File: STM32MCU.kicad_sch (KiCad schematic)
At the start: 5 parts, among them U5 STM32C542CCT6

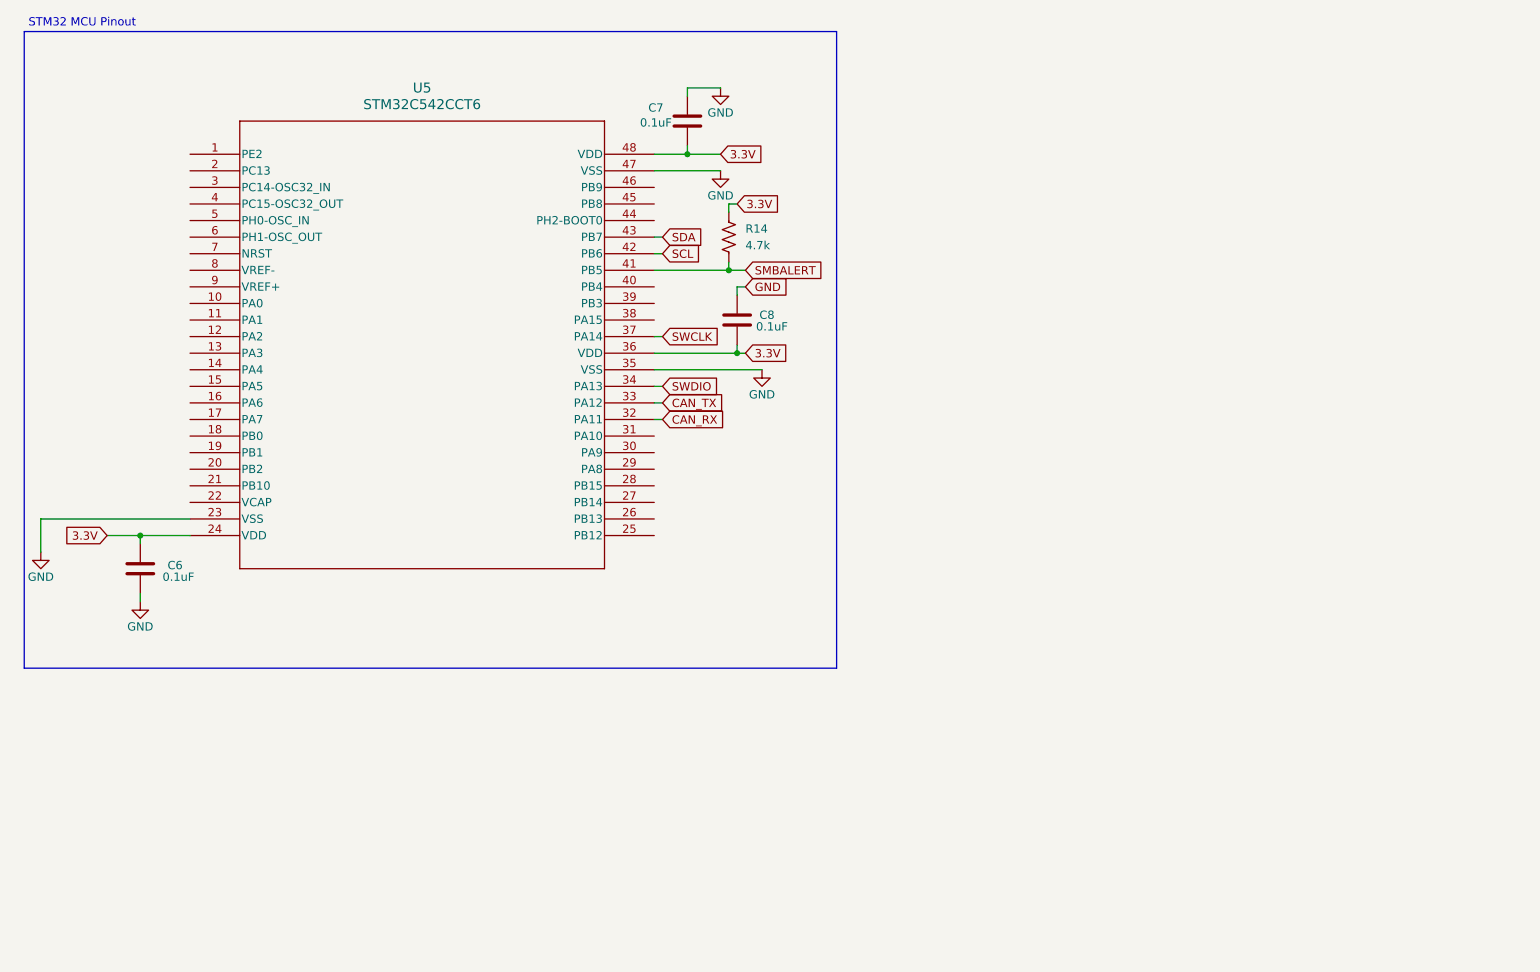
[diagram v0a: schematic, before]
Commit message: Updated MCU
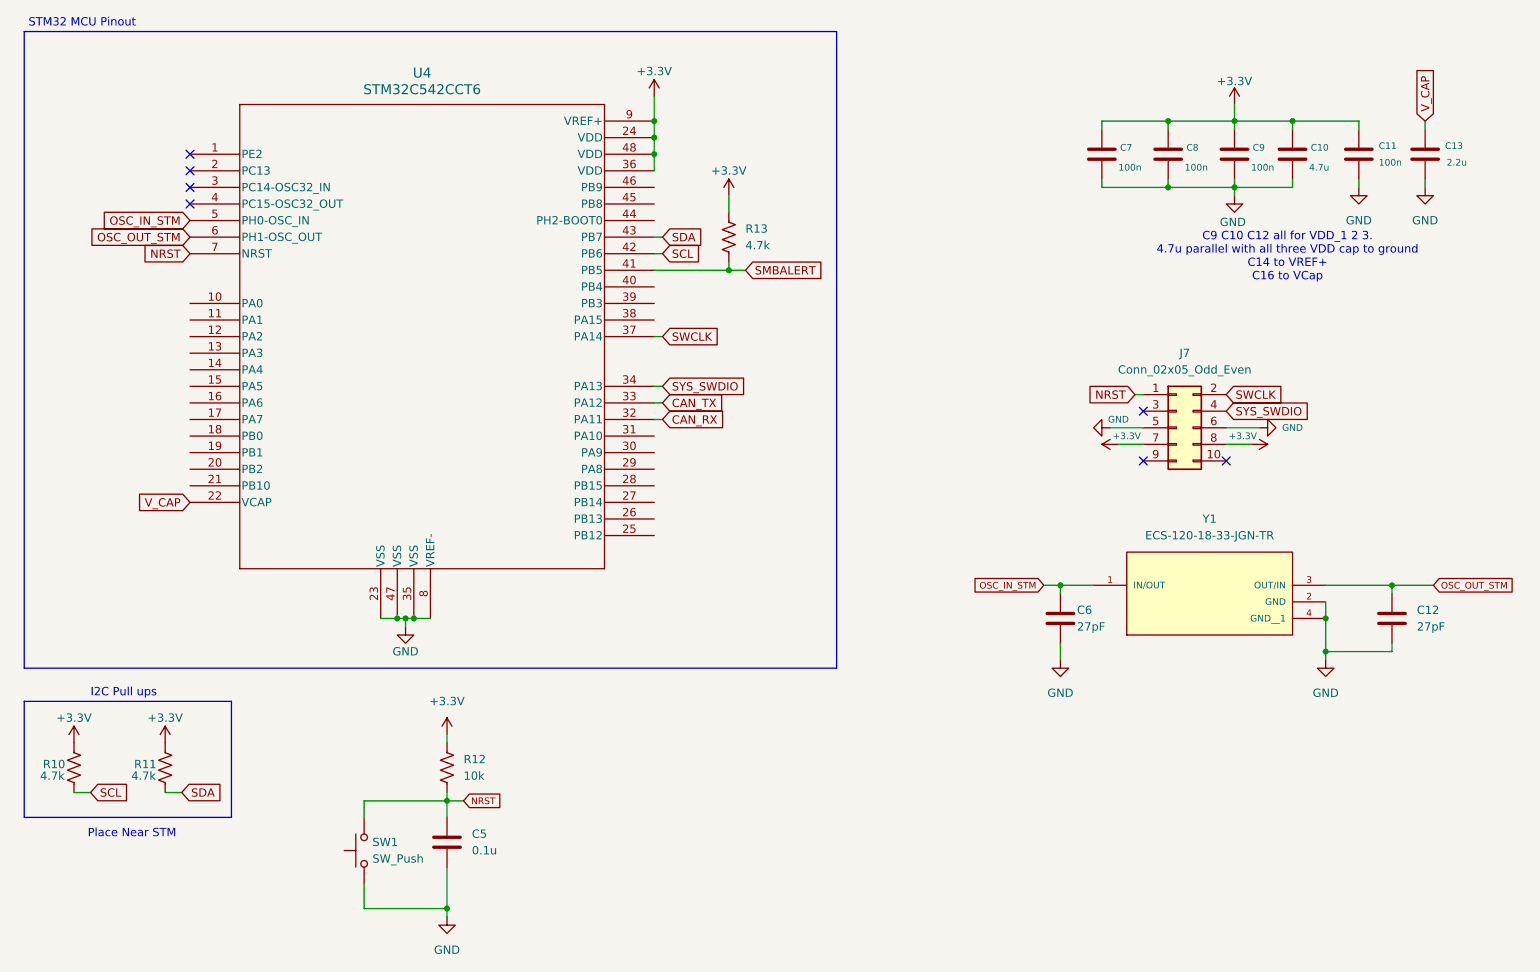
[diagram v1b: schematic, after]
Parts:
- added C10: 4.7u, symbol Device:C
- added C11, C9: 100n, symbol Device:C
- added C12: 27pF, symbol Device:C
- added C13: 2.2u, symbol Device:C
- added C5: 0.1u, symbol Device:C
- added J7: Conn_02x05_Odd_Even, Oscillator:Oscillator_SMD_ECS_2520MV-xxx-xx-4Pin_2.5x2.0mm, symbol Connector_Generic:Conn_02x05_Odd_Even
- added R10, R11: 4.7k, symbol Device:R_US
- added R12: 10k, Resistor_THT:R_Array_SIP4, symbol Device:R_US
- added SW1: SW_Push, Button_Switch_THT:SW_NKK_GW12LJP, symbol Switch:SW_Push
- added Y1: ECS-120-18-33-JGN-TR, ECS-120-18-33-JGN-TR:XTAL_ECS-120-18-33-JGN-TR, symbol ECS-120-18-33-JGN-TR:ECS-120-18-33-JGN-TR
- C6: value 0.1uF -> 27pF; footprint SOT-23-5_MC_MCH -> (none)
- C7, C8: value 0.1uF -> 100n; footprint SOT-23-5_MC_MCH -> (none)
- renumbered R14 to R13, U5 to U4
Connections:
- net GND: now also U4.8 (VREF-), C10.2, C11.2, C12.2, C13.2, C5.2, C9.2, J7.5 (Pin_5), J7.6 (Pin_6), SW1.1, Y1.2 (GND), Y1.4 (GND__1)
- net SCL: now also R10.1
- net SDA: now also R11.1
- net SWCLK: now also J7.2 (Pin_2)
- net V_CAP: now reaches U4.22 (VCAP)
- net V_CAP: now also C13.1
- net OSC_IN_STM: now reaches U4.5 (PH0-OSC_IN)
- net OSC_IN_STM: now also C6.2, Y1.1 (IN/OUT)
- net OSC_OUT_STM: now reaches U4.6 (PH1-OSC_OUT)
- net OSC_OUT_STM: now also C12.1, Y1.3 (OUT/IN)
- net NRST: now reaches U4.7 (NRST)
- net NRST: now also C5.1, J7.1 (Pin_1), R12.2, SW1.2
- net +3.3V: now reaches U4.9 (VREF+)
- net +3.3V: now also C7.1, C8.1, R13.1, U4.24 (VDD), U4.36 (VDD), U4.48 (VDD), C10.1, C11.1, C9.1, J7.7 (Pin_7), J7.8 (Pin_8), R10.2, R11.2, R12.1
- removed net 3.3V: C6.2, C7.1, C8.1, R13.1, U4.24 (VDD), U4.36 (VDD), U4.48 (VDD)
- net SWDIO renamed SYS_SWDIO
- net SYS_SWDIO: now also J7.4 (Pin_4)
- no-connect marks 0 -> 7
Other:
- note added: "C9 C10 C12 all for VDD_1 2 3. 4.7u parallel with all three VDD cap to ground C14 to VREF+ C16 to VCap"
- note added: "I2C Pull ups"
- note added: "Place Near STM"
- moved on the sheet: U4
